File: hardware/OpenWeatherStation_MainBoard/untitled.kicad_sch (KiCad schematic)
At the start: 62 parts, among them Q1 Q_NMOS_GDS, U10 TL431DBV, U5 PM8800A, U6 POE13P-33L, U9 TCMT1107

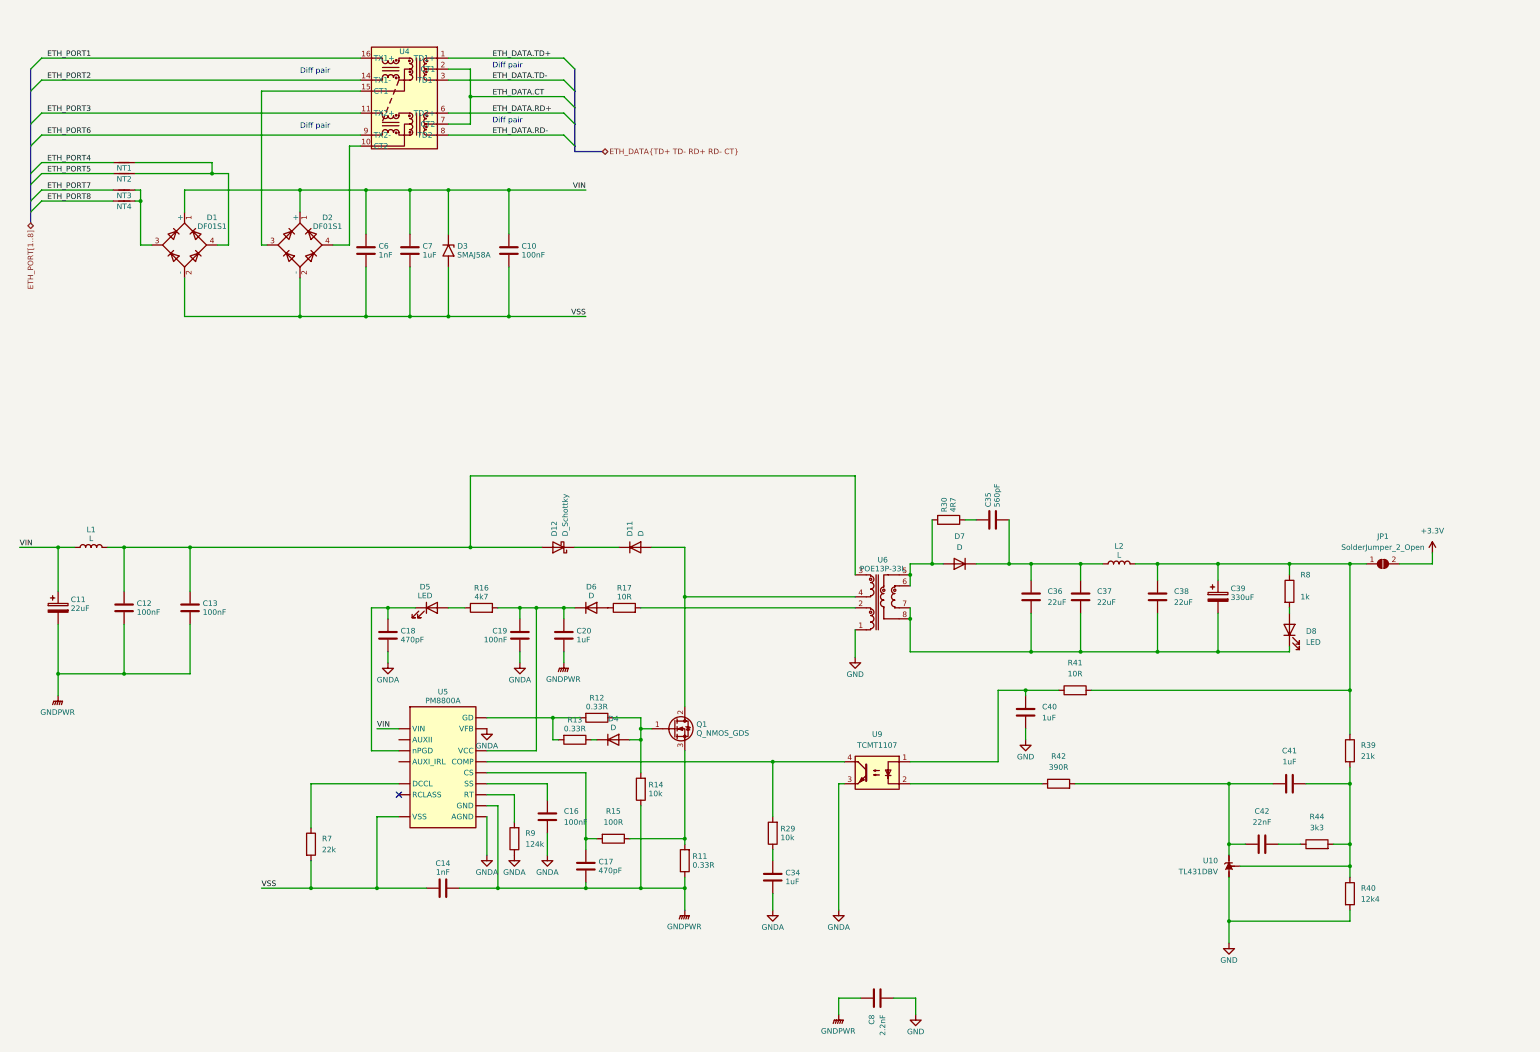
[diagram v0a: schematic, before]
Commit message: update elec
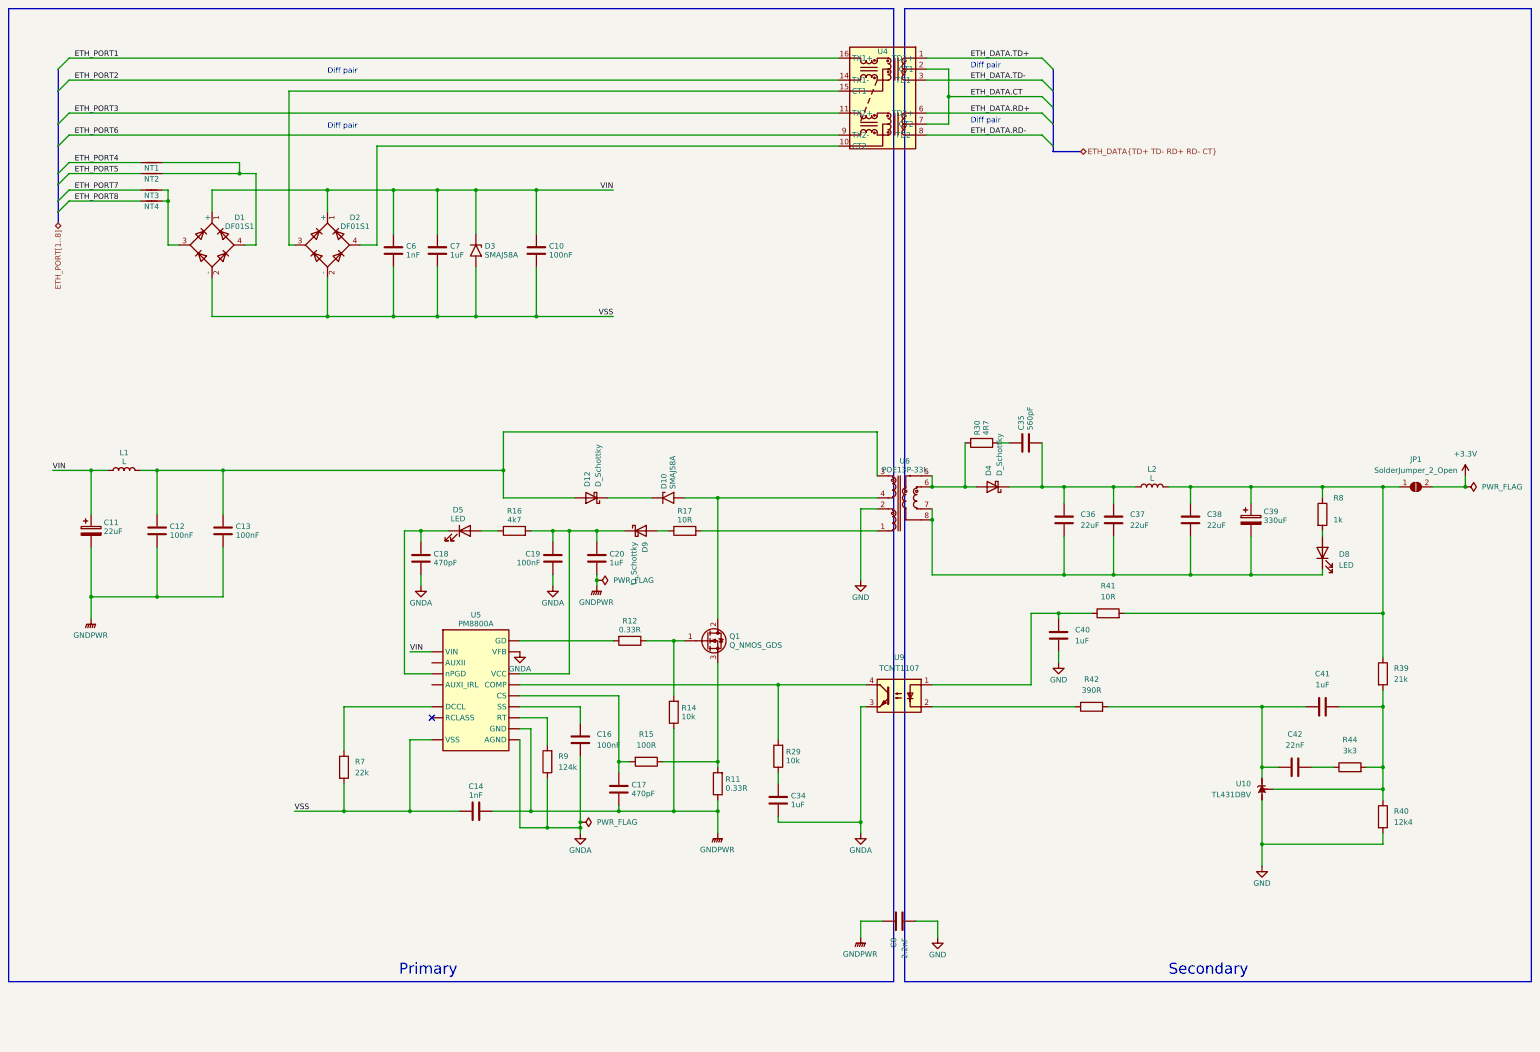
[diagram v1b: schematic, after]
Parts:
- removed D11, D4, D6, D7: D, symbol Device:D
- removed R13: 0.33R, Resistor_SMD:R_0603_1608Metric, symbol Device:R
- added D10: SMAJ58A, Diode_SMD:D_SMA, symbol Diode:SMAJ58A
- added D4, D9: D_Schottky, symbol Device:D_Schottky
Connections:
- net GND: now also U6.2; no longer U6.1
- net at D12.1 (K): now also D10.1 (A1)
- net at Q1.2 (D), U6.4: now also D10.2 (A2)
- net at C19.1, C20.1, R16.2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: now also D9.1 (K)
- net at C35.2, C36.2, C37.2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: now also D4.1 (K)
- net at R17.2: now also U6.1; no longer U6.2
- net at R30.2, U6.5, U6.6: now also D4.2 (A)
- net at R17.1: now also D9.2 (A)
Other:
- note added: "Primary"
- note added: "Secondary"
- moved on the sheet: C10, C11, C12, C13, C14, C16, C17, C18, C19, C20, C34, C35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
